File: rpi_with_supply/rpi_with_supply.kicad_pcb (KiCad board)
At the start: 2 copper layers, 65 x 56 mm, 43 parts, among them IC1 ATTINY85-S, J3 Phoenix 1933189 COMBICON, J4 Phoenix 1933189 COMBICON, J5 Raspberry_Pi_2_3, J6 FAN, P1 CONN_1, P10 CONN_02X02, P11 WS2812, P2 CONN_1, P3 CONN_1, P4 CONN_1, P5 CONN_1, P6 CONN_1, P7 CONN_1, P8 CONN_1, P9 CONN_1, Q1 Q_NMOS_GDS, U1 A8498, U2 L7812, U3 vn7040-switch

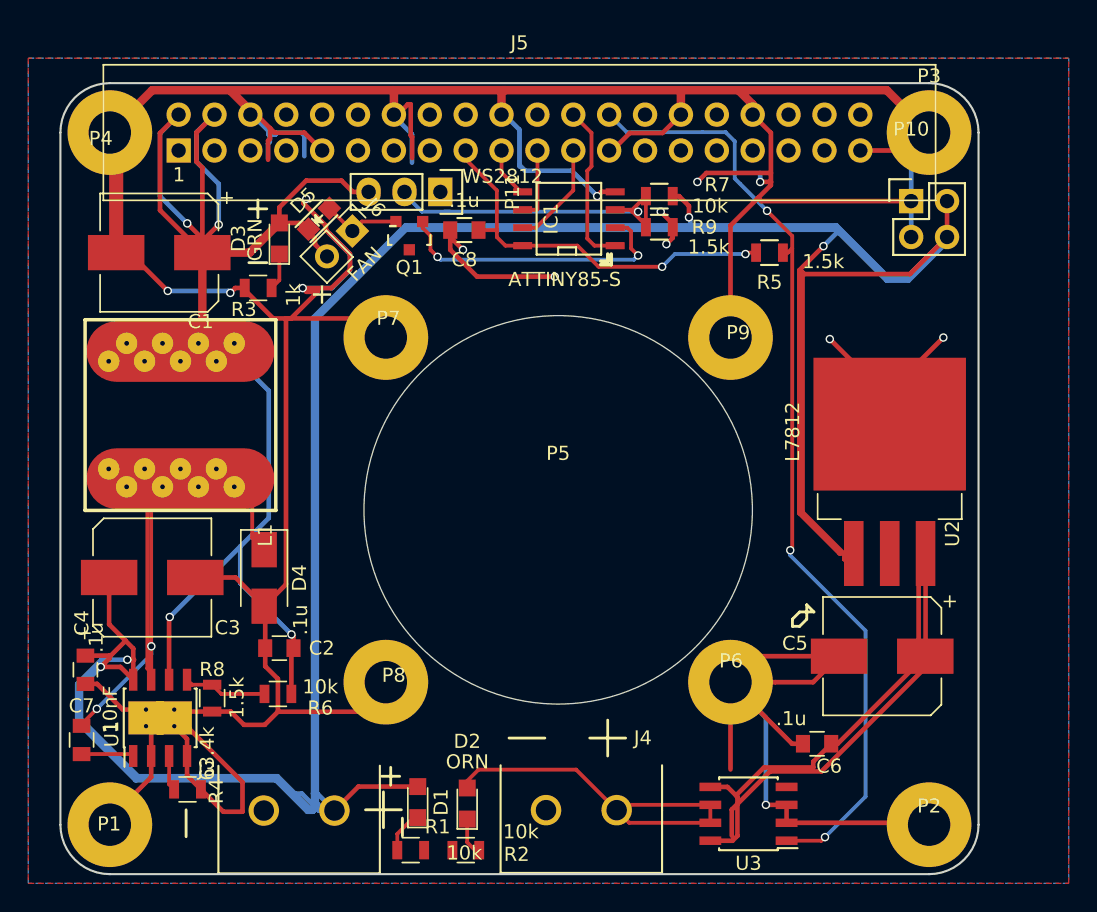
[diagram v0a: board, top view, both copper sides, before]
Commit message: bump
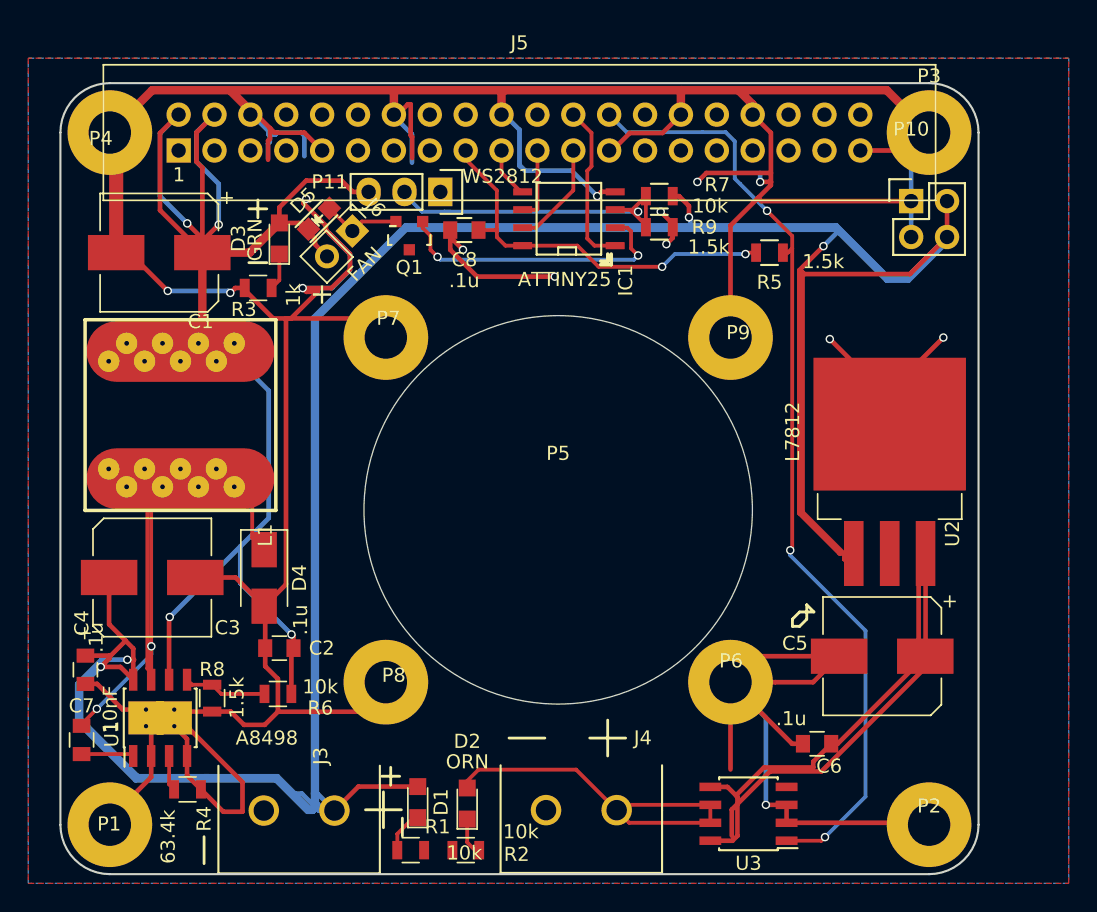
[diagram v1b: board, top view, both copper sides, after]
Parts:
- IC1: value ATTINY85-S -> ATTINY25
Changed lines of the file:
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@@
   (module PHOENIX1933189 (layer F.Cu)
     (at 33.4 68)
-    (fp_text reference J3 (at -6.546 -2.922) (layer F.SilkS)
+    (fp_text reference J3 (at 1.525 -3.865 90) (layer F.SilkS)
       (effects (font (size 1 1) (thickness 0.15)))
     )
@@
     (tags "resistor 0805")
     (attr smd)
-    (fp_text reference R4 (at 2.032 0.127 90) (layer F.SilkS)
-      (effects (font (size 1 1) (thickness 0.15)))
-    )
-    (fp_text value 63.4k (at 1.397 -2.54 90) (layer F.SilkS)
+    (fp_text reference R4 (at 1.17 2.08 270) (layer F.SilkS)
+      (effects (font (size 1 1) (thickness 0.15)))
+    )
+    (fp_text value 63.4k (at -1.37 3.35 90) (layer F.SilkS)
       (effects (font (size 1 1) (thickness 0.15)))
     )
@@
       (effects (font (size 1 1) (thickness 0.15)))
     )
-    (fp_text value A8498 (at 0.381 0.127 180) (layer F.Fab)
+    (fp_text value A8498 (at -1.428 7.554 180) (layer F.SilkS)
       (effects (font (size 1 1) (thickness 0.15)))
     )
@@
       (effects (font (size 1 1) (thickness 0.15)))
     )
-    (fp_text value .1u (at 0 2.1 180) (layer F.SilkS)
+    (fp_text value .1u (at 0.015 -3.58 180) (layer F.SilkS)
       (effects (font (size 1 1) (thickness 0.15)))
     )
@@
     (tags "CMS SOJ")
     (attr smd)
-    (fp_text reference IC1 (at 0 -1.27 90) (layer F.SilkS)
-      (effects (font (size 1 1) (thickness 0.15)))
-    )
-    (fp_text value ATTINY85-S (at -4.3 -0.3 180) (layer F.SilkS)
+    (fp_text reference IC1 (at -4.38 4.015 90) (layer F.SilkS)
+      (effects (font (size 1 1) (thickness 0.15)))
+    )
+    (fp_text value ATTINY25 (at -4.3 -0.3 180) (layer F.SilkS)
       (effects (font (size 1 1) (thickness 0.15)))
     )
@@
       (effects (font (size 1 1) (thickness 0.15)))
     )
-    (fp_text value Q_NMOS_GDS (at 0 2.3 180) (layer F.Fab)
+    (fp_text value Q_NMOS_GDS (at -1.98 -3.815 180) (layer F.Fab)
       (effects (font (size 1 1) (thickness 0.15)))
     )
@@
     (descr "Through hole pin header")
     (tags "pin header")
-    (fp_text reference P11 (at 0 -5.1 270) (layer F.SilkS)
+    (fp_text reference P11 (at -0.705 7.84 360) (layer F.SilkS)
       (effects (font (size 1 1) (thickness 0.15)))
     )
@@
   (gr_line (start 53.975 62.865) (end 56.515 62.865) (angle 90) (layer F.SilkS) (width 0.2))
   (gr_line (start 48.26 62.865) (end 50.8 62.865) (angle 90) (layer F.SilkS) (width 0.2))
-  (gr_line (start 25.4 69.85) (end 25.4 67.945) (angle 90) (layer F.SilkS) (width 0.2))
+  (gr_line (start 26.67 71.755) (end 26.67 69.85) (angle 90) (layer F.SilkS) (width 0.2))
   (gr_line (start 39.37 69.215) (end 39.37 66.675) (angle 90) (layer F.SilkS) (width 0.2))
   (gr_line (start 38.1 67.945) (end 40.64 67.945) (angle 90) (layer F.SilkS) (width 0.2))
